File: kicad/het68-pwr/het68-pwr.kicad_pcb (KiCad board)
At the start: 2 copper layers, 90 x 50 mm, 20 parts, among them J1 AC_IN, J2 USB_C, J3 VSYS_OUT

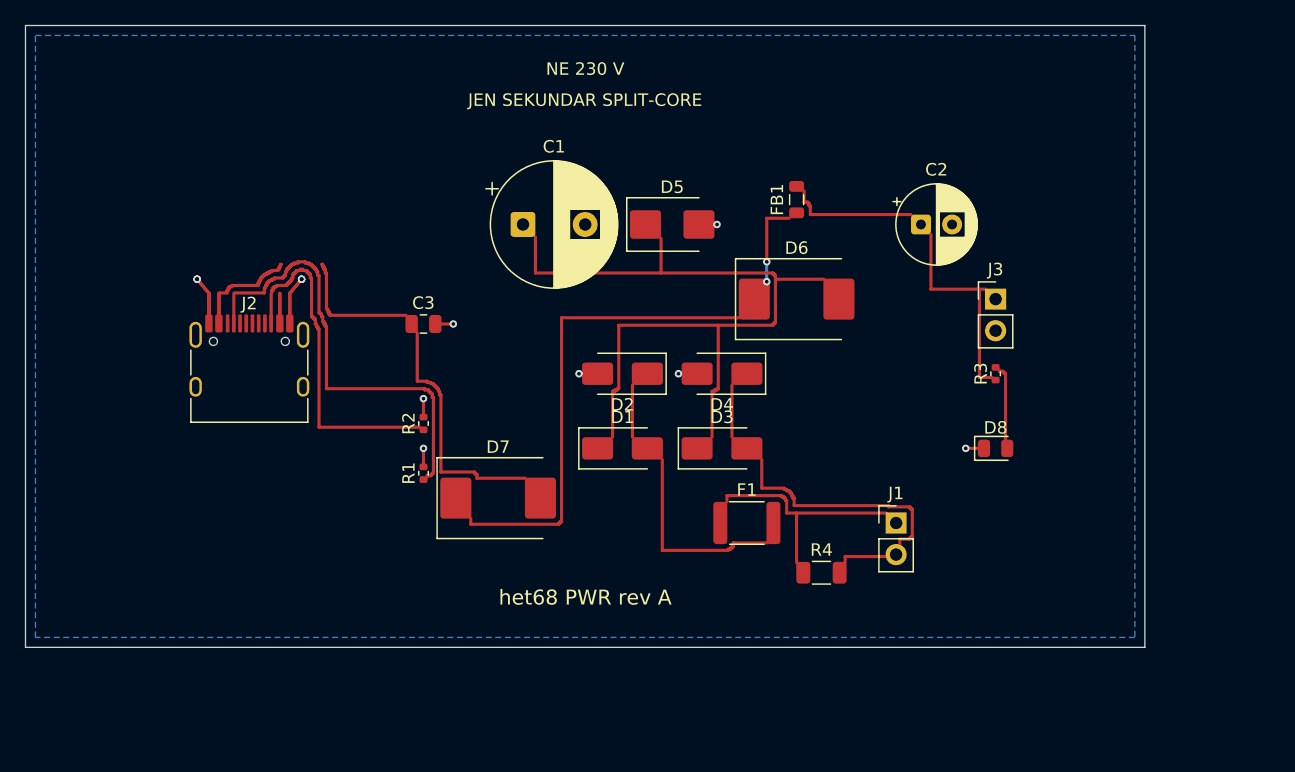
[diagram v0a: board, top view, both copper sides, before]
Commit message: Protect the CT secondary and ship clean power and satellite fab files.
Add burden, LC filter and crowbar on the power board, close DRC on power and satellite, and refresh the board previews for v1.10.0.

Co-authored-by: Cursor <cursoragent@cursor.com>
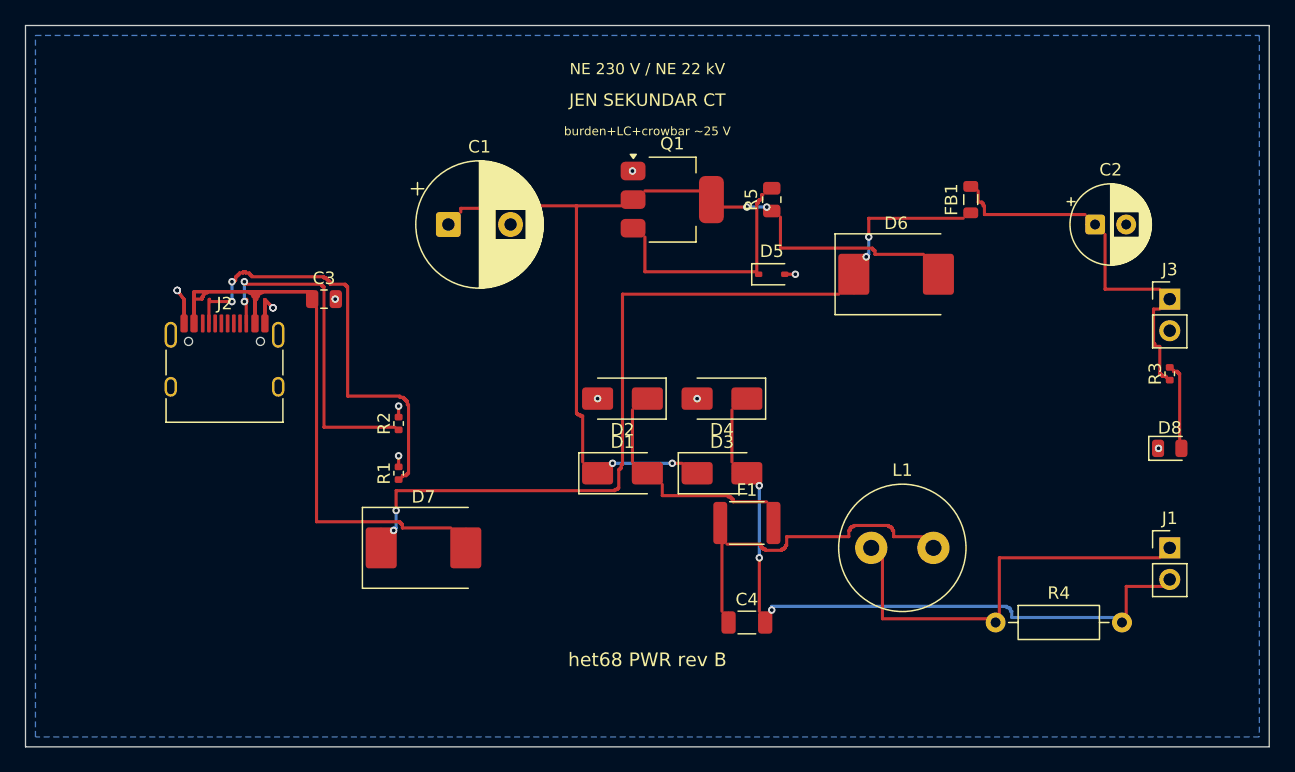
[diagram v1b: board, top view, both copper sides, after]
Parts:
- added C4: 1u/100V, C_1206_3216Metric, F.Cu at (58.0, 48.0)
- added L1: 470uH, L_Radial_D10.0mm_P5.00mm_Fastron_07P, F.Cu at (68.0, 42.0)
- added Q1: X0202MN, SOT-223, F.Cu at (52.0, 14.0)
- added R5: 1k, R_0805_2012Metric, F.Cu at (60.0, 14.0)
- C1: value 470u/25V -> 470u/50V
- D5: value SMBJ15A -> BZX84-C24; footprint D_SMB -> D_SOD-323
- R4: footprint R_1206_3216Metric -> R_Axial_DIN0207_L6.3mm_D2.5mm_P10.16mm_Horizontal
- moved J1 22.1 mm to (92.0, 42.0)
- moved R4 14.6 mm to (78.0, 48.0)
- moved C2 14.0 mm to (86.0, 16.0)
- moved D8 14.0 mm to (92.0, 34.0)
- moved FB1 14.0 mm to (76.0, 14.0)
- moved J3 14.0 mm to (92.0, 22.0)
- moved R3 14.0 mm to (92.0, 28.0)
- moved D5 8.94 mm to (60.0, 20.0)
- moved C3 8.25 mm to (24.0, 22.0)
- moved D6 8.25 mm to (70.0, 20.0)
- moved D7 7.21 mm to (32.0, 42.0)
- moved C1 6.00 mm to (34.0, 16.0)
- moved D1 2.00 mm to (48.0, 36.0)
- moved D2 2.00 mm to (48.0, 30.0)
- moved D3 2.00 mm to (56.0, 36.0)
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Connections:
- D5 pad 1: DC -> SCR_G
- F1 pad 1: AC1 -> AC1L
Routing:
- net VBUS: track 50.4 -> 79.5 mm
- net AC1L: track 0.00 -> 27.9 mm
- net AC2: track 31.6 -> 52.5 mm, vias 0 -> 3
- net VSYS_RAW: track 49.0 -> 69.1 mm, vias 2 -> 4
- net SCR_G: track 0.00 -> 19.9 mm
- net GND: track 25.9 -> 14.0 mm, vias 11 -> 12
- net AC1: track 21.7 -> 33.1 mm
- net AC1F: track 24.2 -> 17.7 mm
- net CC2: track 29.1 -> 27.9 mm, vias 0 -> 2
- net CC1: track 38.9 -> 37.7 mm, vias 0 -> 2
- net VSYS: track 29.4 -> 28.2 mm
- net DC: track 70.3 -> 69.3 mm, vias 0 -> 4
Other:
- board size 90 x 50 mm -> 100 x 58 mm
- board text added: "JEN SEKUNDAR CT"
- board text added: "NE 230 V / NE 22 kV"
- board text added: "burden+LC+crowbar ~25 V"
- board text added: "het68 PWR rev B"
- board text removed: "JEN SEKUNDAR SPLIT-CORE"
- board text removed: "NE 230 V"
- board text removed: "het68 PWR rev A"
